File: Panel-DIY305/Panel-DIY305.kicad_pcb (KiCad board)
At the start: 2 copper layers, 62.2 x 39 mm, 400 parts

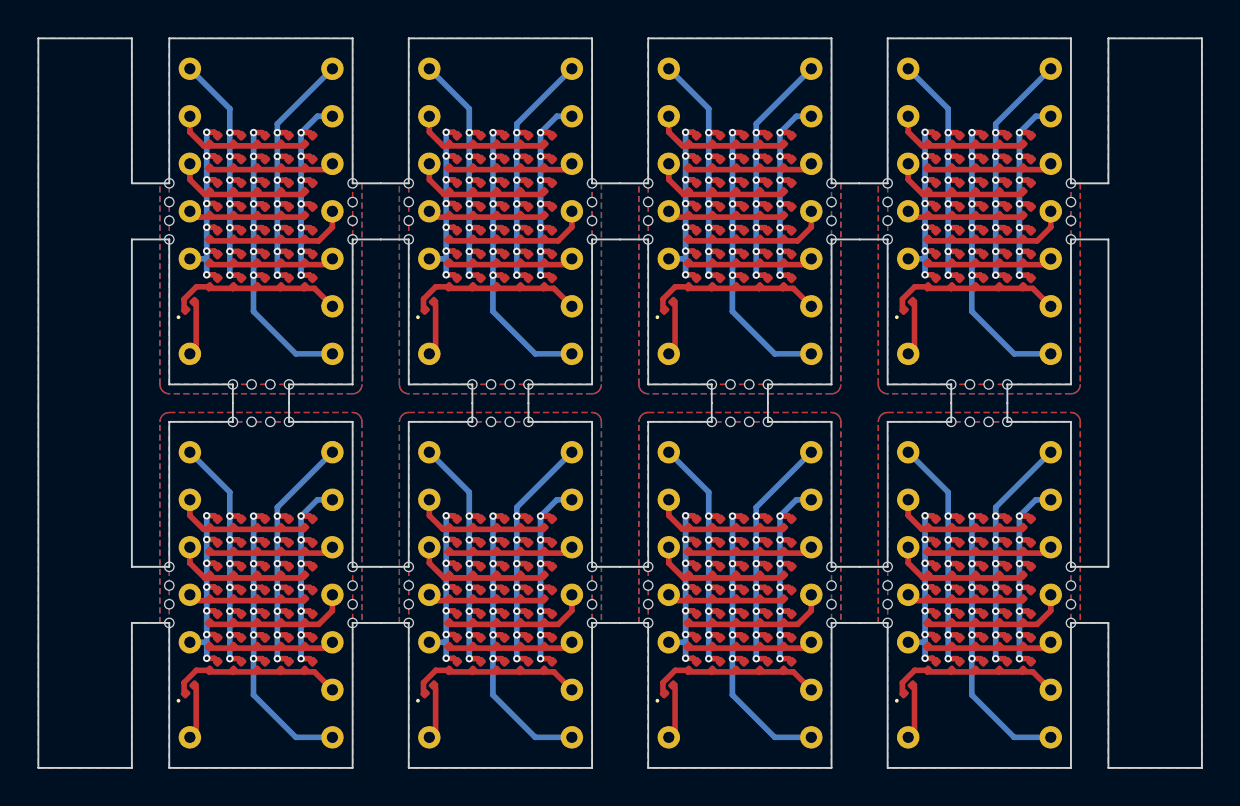
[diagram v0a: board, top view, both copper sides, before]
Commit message: Generated Panel
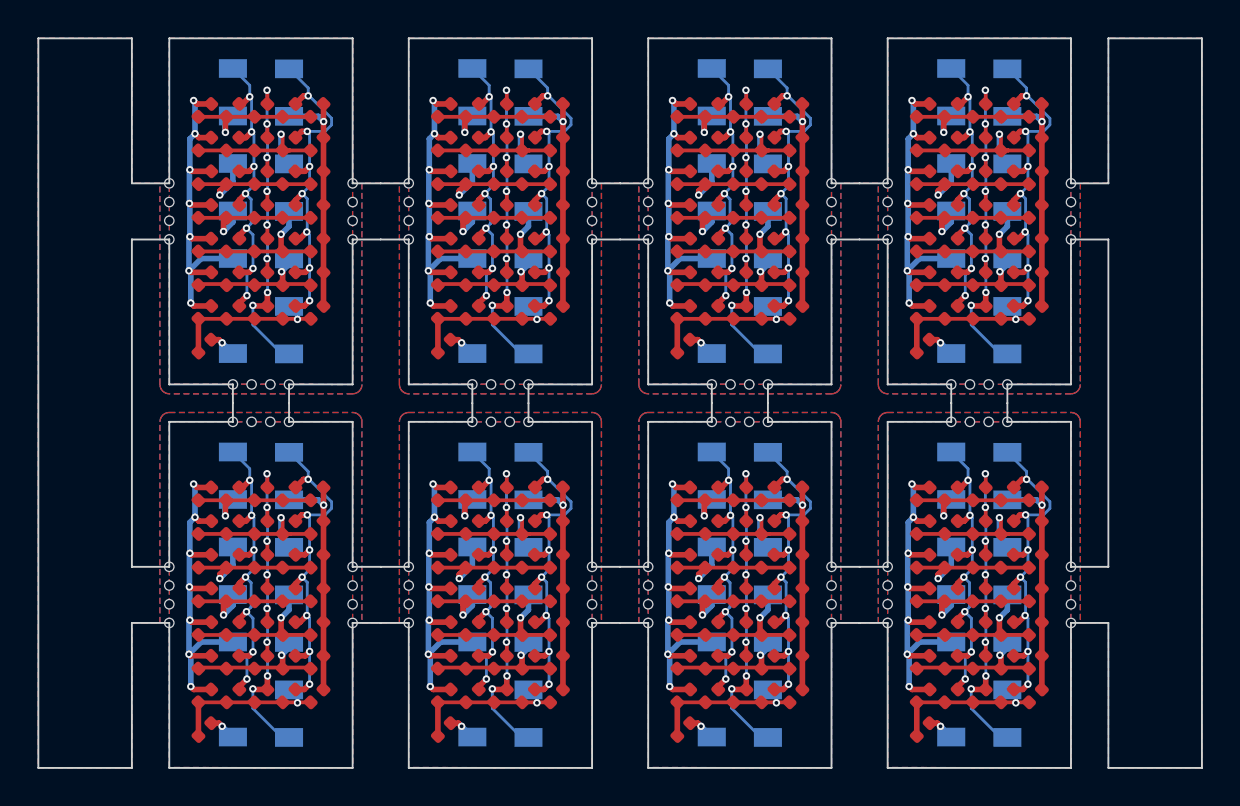
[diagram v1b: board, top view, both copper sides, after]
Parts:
- removed the D1 at (165.2, 25.4)
- removed the D1 at (165.2, 45.9)
- removed the D1 at (126.8, 45.9)
- removed the D1 at (152.4, 25.4)
- removed the D1 at (152.4, 45.9)
- removed the D1 at (139.6, 25.4)
- removed the D1 at (139.6, 45.9)
- removed the D1 at (126.8, 25.4)
- removed the D10 at (140.8, 48.5)
- removed the D10 at (128.0, 28.0)
- removed the D10 at (166.4, 28.0)
- removed the D10 at (153.6, 28.0)
- removed the D10 at (140.8, 28.0)
- removed the D10 at (166.4, 48.5)
- removed the D10 at (153.6, 48.5)
- removed the D10 at (128.0, 48.5)
- removed the D11 at (153.6, 49.7)
- removed the D11 at (166.4, 29.2)
- removed the D11 at (128.0, 29.2)
- removed the D11 at (140.8, 29.2)
- removed the D11 at (128.0, 49.7)
- removed the D11 at (140.8, 49.7)
- removed the D11 at (153.6, 29.2)
- removed the D11 at (166.4, 49.7)
- removed the D12 at (128.0, 30.5)
- removed the D12 at (140.8, 30.5)
- removed the D12 at (153.6, 30.5)
- removed the D12 at (166.4, 30.5)
- removed the D12 at (166.4, 51.0)
- removed the D12 at (140.8, 51.0)
- removed the D12 at (128.0, 51.0)
- removed the D12 at (153.6, 51.0)
- removed the D13 at (166.4, 31.8)
- removed the D13 at (166.4, 52.3)
- removed the D13 at (153.6, 31.8)
- removed the D13 at (140.8, 52.3)
- removed the D13 at (153.6, 52.3)
- removed the D13 at (128.0, 31.8)
- removed the D13 at (128.0, 52.3)
- removed the D13 at (140.8, 31.8)
- removed the D14 at (128.0, 53.6)
- removed the D14 at (153.6, 33.1)
- removed the D14 at (166.4, 53.6)
- removed the D14 at (128.0, 33.1)
- removed the D14 at (153.6, 53.6)
- removed the D14 at (140.8, 53.6)
- removed the D14 at (166.4, 33.1)
- removed the D14 at (140.8, 33.1)
- removed the D15 at (167.7, 25.4)
- removed the D15 at (129.3, 45.9)
- removed the D15 at (154.9, 45.9)
- removed the D15 at (154.9, 25.4)
- removed the D15 at (167.7, 45.9)
- removed the D15 at (142.1, 45.9)
- removed the D15 at (129.3, 25.4)
- removed the D15 at (142.1, 25.4)
- removed the D16 at (154.9, 26.7)
- removed the D16 at (142.1, 26.7)
- removed the D16 at (167.7, 26.7)
- removed the D16 at (129.3, 47.2)
- removed the D16 at (154.9, 47.2)
- removed the D16 at (129.3, 26.7)
- removed the D16 at (167.7, 47.2)
- removed the D16 at (142.1, 47.2)
- removed the D17 at (129.3, 28.0)
- removed the D17 at (167.7, 28.0)
- removed the D17 at (154.9, 28.0)
- removed the D17 at (142.1, 48.5)
- removed the D17 at (167.7, 48.5)
- removed the D17 at (142.1, 28.0)
- removed the D17 at (129.3, 48.5)
- removed the D17 at (154.9, 48.5)
- removed the D18 at (167.7, 49.7)
- removed the D18 at (167.7, 29.2)
- removed the D18 at (129.3, 49.7)
- removed the D18 at (142.1, 49.7)
- removed the D18 at (129.3, 29.2)
- removed the D18 at (142.1, 29.2)
- removed the D18 at (154.9, 29.2)
- removed the D18 at (154.9, 49.7)
- removed the D19 at (142.1, 51.0)
- removed the D19 at (129.3, 51.0)
- removed the D19 at (142.1, 30.5)
- removed the D19 at (167.7, 51.0)
- removed the D19 at (154.9, 51.0)
- removed the D19 at (154.9, 30.5)
- removed the D19 at (129.3, 30.5)
- removed the D19 at (167.7, 30.5)
- removed the D2 at (126.8, 26.7)
- removed the D2 at (126.8, 47.2)
- removed the D2 at (165.2, 26.7)
- removed the D2 at (165.2, 47.2)
- removed the D2 at (139.6, 47.2)
- removed the D2 at (139.6, 26.7)
- removed the D2 at (152.4, 26.7)
- removed the D2 at (152.4, 47.2)
- removed the D20 at (154.9, 31.8)
- removed the D20 at (154.9, 52.3)
- removed the D20 at (167.7, 52.3)
- removed the D20 at (129.3, 31.8)
- removed the D20 at (129.3, 52.3)
- removed the D20 at (142.1, 52.3)
- removed the D20 at (142.1, 31.8)
- removed the D20 at (167.7, 31.8)
- removed the D21 at (154.9, 33.1)
- removed the D21 at (167.7, 33.1)
- removed the D21 at (167.7, 53.6)
- removed the D21 at (129.3, 33.1)
- removed the D21 at (142.1, 53.6)
- removed the D21 at (129.3, 53.6)
- removed the D21 at (154.9, 53.6)
- removed the D21 at (142.1, 33.1)
- removed the D22 at (156.2, 25.4)
- removed the D22 at (143.4, 25.4)
- removed the D22 at (169.0, 25.4)
- removed the D22 at (156.2, 45.9)
- removed the D22 at (130.6, 45.9)
- removed the D22 at (130.6, 25.4)
- removed the D22 at (143.4, 45.9)
- removed the D22 at (169.0, 45.9)
- removed the D23 at (143.4, 26.7)
- removed the D23 at (156.2, 47.2)
- removed the D23 at (143.4, 47.2)
- removed the D23 at (156.2, 26.7)
- removed the D23 at (169.0, 26.7)
- removed the D23 at (169.0, 47.2)
- removed the D23 at (130.6, 47.2)
- removed the D23 at (130.6, 26.7)
- removed the D24 at (130.6, 28.0)
- removed the D24 at (169.0, 48.5)
- removed the D24 at (130.6, 48.5)
- removed the D24 at (143.4, 48.5)
- removed the D24 at (156.2, 28.0)
- removed the D24 at (156.2, 48.5)
- removed the D24 at (143.4, 28.0)
- removed the D24 at (169.0, 28.0)
- removed the D25 at (169.0, 49.7)
- removed the D25 at (156.2, 49.7)
- removed the D25 at (143.4, 49.7)
- removed the D25 at (143.4, 29.2)
- removed the D25 at (130.6, 29.2)
- removed the D25 at (156.2, 29.2)
- removed the D25 at (130.6, 49.7)
- removed the D25 at (169.0, 29.2)
- removed the D26 at (143.4, 30.5)
- removed the D26 at (156.2, 30.5)
- removed the D26 at (130.6, 51.0)
- removed the D26 at (143.4, 51.0)
- removed the D26 at (156.2, 51.0)
- removed the D26 at (169.0, 51.0)
- removed the D26 at (169.0, 30.5)
- removed the D26 at (130.6, 30.5)
- removed the D27 at (156.2, 52.3)
- removed the D27 at (130.6, 52.3)
- removed the D27 at (169.0, 31.8)
- removed the D27 at (130.6, 31.8)
- removed the D27 at (169.0, 52.3)
- removed the D27 at (143.4, 31.8)
- removed the D27 at (156.2, 31.8)
- removed the D27 at (143.4, 52.3)
- removed the D28 at (156.2, 53.6)
- removed the D28 at (130.6, 33.1)
- removed the D28 at (169.0, 53.6)
- removed the D28 at (156.2, 33.1)
- removed the D28 at (130.6, 53.6)
- removed the D28 at (169.0, 33.1)
- removed the D28 at (143.4, 33.1)
- removed the D28 at (143.4, 53.6)
- removed the D29 at (144.7, 45.9)
- removed the D29 at (144.7, 25.4)
- removed the D29 at (157.4, 45.9)
- removed the D29 at (131.8, 45.9)
- removed the D29 at (157.4, 25.4)
- removed the D29 at (131.8, 25.4)
- removed the D29 at (170.2, 25.4)
- removed the D29 at (170.2, 45.9)
- removed the D3 at (126.8, 28.0)
- removed the D3 at (165.2, 28.0)
- removed the D3 at (165.2, 48.5)
- removed the D3 at (152.4, 28.0)
- removed the D3 at (126.8, 48.5)
- removed the D3 at (139.6, 48.5)
- removed the D3 at (139.6, 28.0)
- removed the D3 at (152.4, 48.5)
- removed the D30 at (131.8, 47.2)
- removed the D30 at (170.2, 26.7)
- removed the D30 at (157.4, 26.7)
- removed the D30 at (131.8, 26.7)
- removed the D30 at (144.7, 47.2)
- removed the D30 at (157.4, 47.2)
- removed the D30 at (170.2, 47.2)
- removed the D30 at (144.7, 26.7)
- removed the D31 at (170.2, 48.5)
- removed the D31 at (144.7, 28.0)
- removed the D31 at (170.2, 28.0)
- removed the D31 at (157.4, 48.5)
- removed the D31 at (157.4, 28.0)
- removed the D31 at (144.7, 48.5)
- removed the D31 at (131.8, 48.5)
- removed the D31 at (131.8, 28.0)
- removed the D32 at (144.7, 29.2)
- removed the D32 at (157.4, 49.7)
- removed the D32 at (131.8, 29.2)
- removed the D32 at (157.4, 29.2)
- removed the D32 at (131.8, 49.7)
- removed the D32 at (144.7, 49.7)
- removed the D32 at (170.2, 29.2)
- removed the D32 at (170.2, 49.7)
- removed the D33 at (131.8, 51.0)
- removed the D33 at (144.7, 30.5)
- removed the D33 at (131.8, 30.5)
- removed the D33 at (157.4, 51.0)
- removed the D33 at (157.4, 30.5)
- removed the D33 at (170.2, 51.0)
- removed the D33 at (170.2, 30.5)
- removed the D33 at (144.7, 51.0)
- removed the D34 at (144.7, 52.3)
- removed the D34 at (144.7, 31.8)
- removed the D34 at (157.4, 52.3)
- removed the D34 at (170.2, 31.8)
- removed the D34 at (131.8, 52.3)
- removed the D34 at (131.8, 31.8)
- removed the D34 at (170.2, 52.3)
- removed the D34 at (157.4, 31.8)
- removed the D35 at (144.7, 53.6)
- removed the D35 at (157.4, 33.1)
- removed the D35 at (131.8, 33.1)
- removed the D35 at (144.7, 33.1)
- removed the D35 at (131.8, 53.6)
- removed the D35 at (157.4, 53.6)
- removed the D35 at (170.2, 33.1)
- removed the D35 at (170.2, 53.6)
- removed the D36 at (163.9, 34.3)
- removed the D36 at (151.1, 54.8)
- removed the D36 at (163.9, 54.8)
- removed the D36 at (125.5, 54.8)
- removed the D36 at (138.3, 54.8)
- removed the D36 at (151.1, 34.3)
- removed the D36 at (138.3, 34.3)
- removed the D36 at (125.5, 34.3)
- removed the D4 at (126.8, 29.2)
- removed the D4 at (165.2, 49.7)
- removed the D4 at (152.4, 29.2)
- removed the D4 at (139.6, 29.2)
- removed the D4 at (152.4, 49.7)
- removed the D4 at (165.2, 29.2)
- removed the D4 at (139.6, 49.7)
- removed the D4 at (126.8, 49.7)
- removed the D5 at (139.6, 30.5)
- removed the D5 at (139.6, 51.0)
- removed the D5 at (126.8, 51.0)
- removed the D5 at (152.4, 51.0)
- removed the D5 at (152.4, 30.5)
- removed the D5 at (126.8, 30.5)
- removed the D5 at (165.2, 51.0)
- removed the D5 at (165.2, 30.5)
- removed the D6 at (165.2, 52.3)
- removed the D6 at (152.4, 52.3)
- removed the D6 at (126.8, 31.8)
- removed the D6 at (152.4, 31.8)
- removed the D6 at (126.8, 52.3)
- removed the D6 at (165.2, 31.8)
- removed the D6 at (139.6, 52.3)
- removed the D6 at (139.6, 31.8)
- removed the D7 at (126.8, 33.1)
- removed the D7 at (139.6, 53.6)
- removed the D7 at (165.2, 33.1)
- removed the D7 at (126.8, 53.6)
- removed the D7 at (165.2, 53.6)
- removed the D7 at (139.6, 33.1)
- removed the D7 at (152.4, 33.1)
- removed the D7 at (152.4, 53.6)
- removed the D8 at (153.6, 45.9)
- removed the D8 at (153.6, 25.4)
- removed the D8 at (128.0, 25.4)
- removed the D8 at (140.8, 45.9)
- removed the D8 at (128.0, 45.9)
- removed the D8 at (166.4, 25.4)
- removed the D8 at (166.4, 45.9)
- removed the D8 at (140.8, 25.4)
- removed the D9 at (128.0, 26.7)
- removed the D9 at (166.4, 26.7)
- removed the D9 at (140.8, 26.7)
- removed the D9 at (128.0, 47.2)
- removed the D9 at (153.6, 47.2)
- removed the D9 at (140.8, 47.2)
- removed the D9 at (153.6, 26.7)
- removed the D9 at (166.4, 47.2)
- removed G*** (x8): LOGO, LOGO
- removed J4 (x8): , Package_DIP:DIP-14_W7.62mm
- added D1: LED, LED_SMD:LED_0402_1005Metric, F.Cu at (139.1, 44.4)
- added D1: LED, LED_SMD:LED_0402_1005Metric, F.Cu at (164.7, 44.4)
- added D1: LED, LED_SMD:LED_0402_1005Metric, F.Cu at (151.9, 23.9)
- added D1: LED, LED_SMD:LED_0402_1005Metric, F.Cu at (151.9, 44.4)
- added D1: LED, LED_SMD:LED_0402_1005Metric, F.Cu at (126.3, 23.9)
- added D1: LED, LED_SMD:LED_0402_1005Metric, F.Cu at (126.3, 44.4)
- added D1: LED, LED_SMD:LED_0402_1005Metric, F.Cu at (164.7, 23.9)
- added D1: LED, LED_SMD:LED_0402_1005Metric, F.Cu at (139.1, 23.9)
- added D10: LED, LED_SMD:LED_0402_1005Metric, F.Cu at (166.2, 27.4)
- added D10: LED, LED_SMD:LED_0402_1005Metric, F.Cu at (140.6, 27.4)
- added D10: LED, LED_SMD:LED_0402_1005Metric, F.Cu at (140.6, 48.0)
- added D10: LED, LED_SMD:LED_0402_1005Metric, F.Cu at (166.2, 48.0)
- added D10: LED, LED_SMD:LED_0402_1005Metric, F.Cu at (153.4, 48.0)
- added D10: LED, LED_SMD:LED_0402_1005Metric, F.Cu at (127.8, 27.4)
- added D10: LED, LED_SMD:LED_0402_1005Metric, F.Cu at (153.4, 27.4)
- added D10: LED, LED_SMD:LED_0402_1005Metric, F.Cu at (127.8, 48.0)
- added D11: LED, LED_SMD:LED_0402_1005Metric, F.Cu at (140.6, 29.2)
- added D11: LED, LED_SMD:LED_0402_1005Metric, F.Cu at (140.6, 49.8)
- added D11: LED, LED_SMD:LED_0402_1005Metric, F.Cu at (153.4, 29.2)
- added D11: LED, LED_SMD:LED_0402_1005Metric, F.Cu at (127.8, 49.8)
- added D11: LED, LED_SMD:LED_0402_1005Metric, F.Cu at (153.4, 49.8)
- added D11: LED, LED_SMD:LED_0402_1005Metric, F.Cu at (166.2, 49.8)
- added D11: LED, LED_SMD:LED_0402_1005Metric, F.Cu at (166.2, 29.2)
- added D11: LED, LED_SMD:LED_0402_1005Metric, F.Cu at (127.8, 29.2)
- added D12: LED, LED_SMD:LED_0402_1005Metric, F.Cu at (166.2, 51.5)
- added D12: LED, LED_SMD:LED_0402_1005Metric, F.Cu at (140.6, 51.5)
- added D12: LED, LED_SMD:LED_0402_1005Metric, F.Cu at (140.6, 31.1)
- added D12: LED, LED_SMD:LED_0402_1005Metric, F.Cu at (153.4, 51.5)
- added D12: LED, LED_SMD:LED_0402_1005Metric, F.Cu at (166.2, 31.1)
- added D12: LED, LED_SMD:LED_0402_1005Metric, F.Cu at (153.4, 31.1)
- added D12: LED, LED_SMD:LED_0402_1005Metric, F.Cu at (127.8, 51.5)
- added D12: LED, LED_SMD:LED_0402_1005Metric, F.Cu at (127.8, 31.1)
- added D13: LED, LED_SMD:LED_0402_1005Metric, F.Cu at (166.2, 53.4)
- added D13: LED, LED_SMD:LED_0402_1005Metric, F.Cu at (140.6, 53.4)
- added D13: LED, LED_SMD:LED_0402_1005Metric, F.Cu at (166.2, 32.9)
- added D13: LED, LED_SMD:LED_0402_1005Metric, F.Cu at (127.8, 32.9)
- added D13: LED, LED_SMD:LED_0402_1005Metric, F.Cu at (153.4, 53.4)
- added D13: LED, LED_SMD:LED_0402_1005Metric, F.Cu at (127.8, 53.4)
- added D13: LED, LED_SMD:LED_0402_1005Metric, F.Cu at (140.6, 32.9)
- added D13: LED, LED_SMD:LED_0402_1005Metric, F.Cu at (153.4, 32.9)
- added D14: LED, LED_SMD:LED_0402_1005Metric, F.Cu at (127.8, 55.1)
- added D14: LED, LED_SMD:LED_0402_1005Metric, F.Cu at (140.6, 34.6)
- added D14: LED, LED_SMD:LED_0402_1005Metric, F.Cu at (127.8, 34.6)
- added D14: LED, LED_SMD:LED_0402_1005Metric, F.Cu at (166.2, 55.1)
- added D14: LED, LED_SMD:LED_0402_1005Metric, F.Cu at (140.6, 55.1)
- added D14: LED, LED_SMD:LED_0402_1005Metric, F.Cu at (166.2, 34.6)
- added D14: LED, LED_SMD:LED_0402_1005Metric, F.Cu at (153.4, 55.1)
- added D14: LED, LED_SMD:LED_0402_1005Metric, F.Cu at (153.4, 34.6)
- added D15: LED, LED_SMD:LED_0402_1005Metric, F.Cu at (167.7, 44.4)
- added D15: LED, LED_SMD:LED_0402_1005Metric, F.Cu at (142.1, 23.9)
- added D15: LED, LED_SMD:LED_0402_1005Metric, F.Cu at (129.3, 44.4)
- added D15: LED, LED_SMD:LED_0402_1005Metric, F.Cu at (129.3, 23.9)
- added D15: LED, LED_SMD:LED_0402_1005Metric, F.Cu at (154.9, 23.9)
- added D15: LED, LED_SMD:LED_0402_1005Metric, F.Cu at (154.9, 44.4)
- added D15: LED, LED_SMD:LED_0402_1005Metric, F.Cu at (167.7, 23.9)
- added D15: LED, LED_SMD:LED_0402_1005Metric, F.Cu at (142.1, 44.4)
- added D16: LED, LED_SMD:LED_0402_1005Metric, F.Cu at (154.9, 25.6)
- added D16: LED, LED_SMD:LED_0402_1005Metric, F.Cu at (129.3, 46.1)
- added D16: LED, LED_SMD:LED_0402_1005Metric, F.Cu at (142.1, 46.1)
- added D16: LED, LED_SMD:LED_0402_1005Metric, F.Cu at (129.3, 25.6)
- added D16: LED, LED_SMD:LED_0402_1005Metric, F.Cu at (167.7, 46.1)
- added D16: LED, LED_SMD:LED_0402_1005Metric, F.Cu at (167.7, 25.6)
- added D16: LED, LED_SMD:LED_0402_1005Metric, F.Cu at (154.9, 46.1)
- added D16: LED, LED_SMD:LED_0402_1005Metric, F.Cu at (142.1, 25.6)
- added D17: LED, LED_SMD:LED_0402_1005Metric, F.Cu at (129.3, 48.0)
- added D17: LED, LED_SMD:LED_0402_1005Metric, F.Cu at (154.9, 27.4)
- added D17: LED, LED_SMD:LED_0402_1005Metric, F.Cu at (167.7, 48.0)
- added D17: LED, LED_SMD:LED_0402_1005Metric, F.Cu at (154.9, 48.0)
- added D17: LED, LED_SMD:LED_0402_1005Metric, F.Cu at (129.3, 27.4)
- added D17: LED, LED_SMD:LED_0402_1005Metric, F.Cu at (167.7, 27.4)
- added D17: LED, LED_SMD:LED_0402_1005Metric, F.Cu at (142.1, 48.0)
- added D17: LED, LED_SMD:LED_0402_1005Metric, F.Cu at (142.1, 27.4)
- added D18: LED, LED_SMD:LED_0402_1005Metric, F.Cu at (142.1, 29.2)
- added D18: LED, LED_SMD:LED_0402_1005Metric, F.Cu at (167.7, 49.8)
- added D18: LED, LED_SMD:LED_0402_1005Metric, F.Cu at (129.3, 29.2)
- added D18: LED, LED_SMD:LED_0402_1005Metric, F.Cu at (167.7, 29.2)
- added D18: LED, LED_SMD:LED_0402_1005Metric, F.Cu at (142.1, 49.8)
- added D18: LED, LED_SMD:LED_0402_1005Metric, F.Cu at (154.9, 49.8)
- added D18: LED, LED_SMD:LED_0402_1005Metric, F.Cu at (154.9, 29.2)
- added D18: LED, LED_SMD:LED_0402_1005Metric, F.Cu at (129.3, 49.8)
- added D19: LED, LED_SMD:LED_0402_1005Metric, F.Cu at (167.7, 51.5)
- added D19: LED, LED_SMD:LED_0402_1005Metric, F.Cu at (129.3, 31.1)
- added D19: LED, LED_SMD:LED_0402_1005Metric, F.Cu at (142.1, 51.5)
- added D19: LED, LED_SMD:LED_0402_1005Metric, F.Cu at (167.7, 31.1)
- added D19: LED, LED_SMD:LED_0402_1005Metric, F.Cu at (142.1, 31.1)
- added D19: LED, LED_SMD:LED_0402_1005Metric, F.Cu at (129.3, 51.5)
- added D19: LED, LED_SMD:LED_0402_1005Metric, F.Cu at (154.9, 51.5)
- added D19: LED, LED_SMD:LED_0402_1005Metric, F.Cu at (154.9, 31.1)
- added D2: LED, LED_SMD:LED_0402_1005Metric, F.Cu at (126.3, 25.6)
- added D2: LED, LED_SMD:LED_0402_1005Metric, F.Cu at (151.9, 46.1)
- added D2: LED, LED_SMD:LED_0402_1005Metric, F.Cu at (164.7, 46.1)
- added D2: LED, LED_SMD:LED_0402_1005Metric, F.Cu at (126.3, 46.1)
- added D2: LED, LED_SMD:LED_0402_1005Metric, F.Cu at (151.9, 25.6)
- added D2: LED, LED_SMD:LED_0402_1005Metric, F.Cu at (139.1, 25.6)
- added D2: LED, LED_SMD:LED_0402_1005Metric, F.Cu at (164.7, 25.6)
- added D2: LED, LED_SMD:LED_0402_1005Metric, F.Cu at (139.1, 46.1)
- added D20: LED, LED_SMD:LED_0402_1005Metric, F.Cu at (142.1, 32.9)
- added D20: LED, LED_SMD:LED_0402_1005Metric, F.Cu at (154.9, 32.9)
- added D20: LED, LED_SMD:LED_0402_1005Metric, F.Cu at (129.3, 53.4)
- added D20: LED, LED_SMD:LED_0402_1005Metric, F.Cu at (154.9, 53.4)
- added D20: LED, LED_SMD:LED_0402_1005Metric, F.Cu at (129.3, 32.9)
- added D20: LED, LED_SMD:LED_0402_1005Metric, F.Cu at (167.7, 53.4)
- added D20: LED, LED_SMD:LED_0402_1005Metric, F.Cu at (142.1, 53.4)
- added D20: LED, LED_SMD:LED_0402_1005Metric, F.Cu at (167.7, 32.9)
- added D21: LED, LED_SMD:LED_0402_1005Metric, F.Cu at (167.7, 55.1)
- added D21: LED, LED_SMD:LED_0402_1005Metric, F.Cu at (167.7, 34.6)
- added D21: LED, LED_SMD:LED_0402_1005Metric, F.Cu at (142.1, 34.6)
- added D21: LED, LED_SMD:LED_0402_1005Metric, F.Cu at (129.3, 34.6)
- added D21: LED, LED_SMD:LED_0402_1005Metric, F.Cu at (129.3, 55.1)
- added D21: LED, LED_SMD:LED_0402_1005Metric, F.Cu at (154.9, 34.6)
- added D21: LED, LED_SMD:LED_0402_1005Metric, F.Cu at (154.9, 55.1)
- added D21: LED, LED_SMD:LED_0402_1005Metric, F.Cu at (142.1, 55.1)
- added D22: LED, LED_SMD:LED_0402_1005Metric, F.Cu at (130.8, 23.9)
- added D22: LED, LED_SMD:LED_0402_1005Metric, F.Cu at (143.6, 44.4)
- added D22: LED, LED_SMD:LED_0402_1005Metric, F.Cu at (169.2, 44.4)
- added D22: LED, LED_SMD:LED_0402_1005Metric, F.Cu at (130.8, 44.4)
- added D22: LED, LED_SMD:LED_0402_1005Metric, F.Cu at (156.4, 23.9)
- added D22: LED, LED_SMD:LED_0402_1005Metric, F.Cu at (169.2, 23.9)
- added D22: LED, LED_SMD:LED_0402_1005Metric, F.Cu at (143.6, 23.9)
- added D22: LED, LED_SMD:LED_0402_1005Metric, F.Cu at (156.4, 44.4)
- added D23: LED, LED_SMD:LED_0402_1005Metric, F.Cu at (143.6, 25.6)
- added D23: LED, LED_SMD:LED_0402_1005Metric, F.Cu at (156.4, 46.1)
- added D23: LED, LED_SMD:LED_0402_1005Metric, F.Cu at (130.8, 46.1)
- added D23: LED, LED_SMD:LED_0402_1005Metric, F.Cu at (130.8, 25.6)
- added D23: LED, LED_SMD:LED_0402_1005Metric, F.Cu at (143.6, 46.1)
- added D23: LED, LED_SMD:LED_0402_1005Metric, F.Cu at (169.2, 46.1)
- added D23: LED, LED_SMD:LED_0402_1005Metric, F.Cu at (169.2, 25.6)
- added D23: LED, LED_SMD:LED_0402_1005Metric, F.Cu at (156.4, 25.6)
- added D24: LED, LED_SMD:LED_0402_1005Metric, F.Cu at (156.4, 48.0)
- added D24: LED, LED_SMD:LED_0402_1005Metric, F.Cu at (143.6, 27.4)
- added D24: LED, LED_SMD:LED_0402_1005Metric, F.Cu at (143.6, 48.0)
- added D24: LED, LED_SMD:LED_0402_1005Metric, F.Cu at (130.8, 27.4)
- added D24: LED, LED_SMD:LED_0402_1005Metric, F.Cu at (169.2, 48.0)
- added D24: LED, LED_SMD:LED_0402_1005Metric, F.Cu at (169.2, 27.4)
- added D24: LED, LED_SMD:LED_0402_1005Metric, F.Cu at (156.4, 27.4)
- added D24: LED, LED_SMD:LED_0402_1005Metric, F.Cu at (130.8, 48.0)
- added D25: LED, LED_SMD:LED_0402_1005Metric, F.Cu at (130.8, 29.2)
- added D25: LED, LED_SMD:LED_0402_1005Metric, F.Cu at (156.4, 49.8)
- added D25: LED, LED_SMD:LED_0402_1005Metric, F.Cu at (143.6, 29.2)
- added D25: LED, LED_SMD:LED_0402_1005Metric, F.Cu at (143.6, 49.8)
- added D25: LED, LED_SMD:LED_0402_1005Metric, F.Cu at (169.2, 29.2)
- added D25: LED, LED_SMD:LED_0402_1005Metric, F.Cu at (156.4, 29.2)
- added D25: LED, LED_SMD:LED_0402_1005Metric, F.Cu at (130.8, 49.8)
- added D25: LED, LED_SMD:LED_0402_1005Metric, F.Cu at (169.2, 49.8)
- added D26: LED, LED_SMD:LED_0402_1005Metric, F.Cu at (156.4, 51.5)
- added D26: LED, LED_SMD:LED_0402_1005Metric, F.Cu at (143.6, 51.5)
- added D26: LED, LED_SMD:LED_0402_1005Metric, F.Cu at (156.4, 31.1)
- added D26: LED, LED_SMD:LED_0402_1005Metric, F.Cu at (130.8, 31.1)
- added D26: LED, LED_SMD:LED_0402_1005Metric, F.Cu at (169.2, 31.1)
- added D26: LED, LED_SMD:LED_0402_1005Metric, F.Cu at (130.8, 51.5)
- added D26: LED, LED_SMD:LED_0402_1005Metric, F.Cu at (169.2, 51.5)
- added D26: LED, LED_SMD:LED_0402_1005Metric, F.Cu at (143.6, 31.1)
- added D27: LED, LED_SMD:LED_0402_1005Metric, F.Cu at (156.4, 32.9)
- added D27: LED, LED_SMD:LED_0402_1005Metric, F.Cu at (169.2, 53.4)
- added D27: LED, LED_SMD:LED_0402_1005Metric, F.Cu at (143.6, 53.4)
- added D27: LED, LED_SMD:LED_0402_1005Metric, F.Cu at (130.8, 53.4)
- added D27: LED, LED_SMD:LED_0402_1005Metric, F.Cu at (156.4, 53.4)
- added D27: LED, LED_SMD:LED_0402_1005Metric, F.Cu at (169.2, 32.9)
- added D27: LED, LED_SMD:LED_0402_1005Metric, F.Cu at (143.6, 32.9)
- added D27: LED, LED_SMD:LED_0402_1005Metric, F.Cu at (130.8, 32.9)
- added D28: LED, LED_SMD:LED_0402_1005Metric, F.Cu at (130.8, 34.6)
- added D28: LED, LED_SMD:LED_0402_1005Metric, F.Cu at (156.4, 55.1)
- added D28: LED, LED_SMD:LED_0402_1005Metric, F.Cu at (143.6, 55.1)
- added D28: LED, LED_SMD:LED_0402_1005Metric, F.Cu at (169.2, 34.6)
- added D28: LED, LED_SMD:LED_0402_1005Metric, F.Cu at (169.2, 55.1)
- added D28: LED, LED_SMD:LED_0402_1005Metric, F.Cu at (130.8, 55.1)
- added D28: LED, LED_SMD:LED_0402_1005Metric, F.Cu at (143.6, 34.6)
- added D28: LED, LED_SMD:LED_0402_1005Metric, F.Cu at (156.4, 34.6)
- added D29: LED, LED_SMD:LED_0402_1005Metric, F.Cu at (157.9, 23.9)
- added D29: LED, LED_SMD:LED_0402_1005Metric, F.Cu at (145.1, 44.4)
- added D29: LED, LED_SMD:LED_0402_1005Metric, F.Cu at (145.1, 23.9)
- added D29: LED, LED_SMD:LED_0402_1005Metric, F.Cu at (157.9, 44.4)
- added D29: LED, LED_SMD:LED_0402_1005Metric, F.Cu at (132.3, 44.4)
- added D29: LED, LED_SMD:LED_0402_1005Metric, F.Cu at (132.3, 23.9)
- added D29: LED, LED_SMD:LED_0402_1005Metric, F.Cu at (170.7, 23.9)
- added D29: LED, LED_SMD:LED_0402_1005Metric, F.Cu at (170.7, 44.4)
- added D3: LED, LED_SMD:LED_0402_1005Metric, F.Cu at (164.7, 48.0)
- added D3: LED, LED_SMD:LED_0402_1005Metric, F.Cu at (126.3, 27.4)
- added D3: LED, LED_SMD:LED_0402_1005Metric, F.Cu at (126.3, 48.0)
- added D3: LED, LED_SMD:LED_0402_1005Metric, F.Cu at (139.1, 27.4)
- added D3: LED, LED_SMD:LED_0402_1005Metric, F.Cu at (164.7, 27.4)
- added D3: LED, LED_SMD:LED_0402_1005Metric, F.Cu at (151.9, 48.0)
- added D3: LED, LED_SMD:LED_0402_1005Metric, F.Cu at (139.1, 48.0)
- added D3: LED, LED_SMD:LED_0402_1005Metric, F.Cu at (151.9, 27.4)
- added D30: LED, LED_SMD:LED_0402_1005Metric, F.Cu at (132.3, 46.1)
- added D30: LED, LED_SMD:LED_0402_1005Metric, F.Cu at (157.9, 46.1)
- added D30: LED, LED_SMD:LED_0402_1005Metric, F.Cu at (145.1, 25.6)
- added D30: LED, LED_SMD:LED_0402_1005Metric, F.Cu at (132.3, 25.6)
- added D30: LED, LED_SMD:LED_0402_1005Metric, F.Cu at (145.1, 46.1)
- added D30: LED, LED_SMD:LED_0402_1005Metric, F.Cu at (170.7, 25.6)
- added D30: LED, LED_SMD:LED_0402_1005Metric, F.Cu at (157.9, 25.6)
- added D30: LED, LED_SMD:LED_0402_1005Metric, F.Cu at (170.7, 46.1)
- added D31: LED, LED_SMD:LED_0402_1005Metric, F.Cu at (132.3, 48.0)
- added D31: LED, LED_SMD:LED_0402_1005Metric, F.Cu at (157.9, 27.4)
- added D31: LED, LED_SMD:LED_0402_1005Metric, F.Cu at (145.1, 48.0)
- added D31: LED, LED_SMD:LED_0402_1005Metric, F.Cu at (170.7, 48.0)
- added D31: LED, LED_SMD:LED_0402_1005Metric, F.Cu at (157.9, 48.0)
- added D31: LED, LED_SMD:LED_0402_1005Metric, F.Cu at (170.7, 27.4)
- added D31: LED, LED_SMD:LED_0402_1005Metric, F.Cu at (132.3, 27.4)
- added D31: LED, LED_SMD:LED_0402_1005Metric, F.Cu at (145.1, 27.4)
- added D32: LED, LED_SMD:LED_0402_1005Metric, F.Cu at (145.1, 49.8)
- added D32: LED, LED_SMD:LED_0402_1005Metric, F.Cu at (145.1, 29.2)
- added D32: LED, LED_SMD:LED_0402_1005Metric, F.Cu at (170.7, 49.8)
- added D32: LED, LED_SMD:LED_0402_1005Metric, F.Cu at (132.3, 29.2)
- added D32: LED, LED_SMD:LED_0402_1005Metric, F.Cu at (157.9, 49.8)
- added D32: LED, LED_SMD:LED_0402_1005Metric, F.Cu at (157.9, 29.2)
- added D32: LED, LED_SMD:LED_0402_1005Metric, F.Cu at (132.3, 49.8)
- added D32: LED, LED_SMD:LED_0402_1005Metric, F.Cu at (170.7, 29.2)
- added D33: LED, LED_SMD:LED_0402_1005Metric, F.Cu at (145.1, 51.5)
- added D33: LED, LED_SMD:LED_0402_1005Metric, F.Cu at (157.9, 31.1)
- added D33: LED, LED_SMD:LED_0402_1005Metric, F.Cu at (170.7, 51.5)
- added D33: LED, LED_SMD:LED_0402_1005Metric, F.Cu at (132.3, 31.1)
- added D33: LED, LED_SMD:LED_0402_1005Metric, F.Cu at (170.7, 31.1)
- added D33: LED, LED_SMD:LED_0402_1005Metric, F.Cu at (132.3, 51.5)
- added D33: LED, LED_SMD:LED_0402_1005Metric, F.Cu at (145.1, 31.1)
- added D33: LED, LED_SMD:LED_0402_1005Metric, F.Cu at (157.9, 51.5)
- added D34: LED, LED_SMD:LED_0402_1005Metric, F.Cu at (145.1, 32.9)
- added D34: LED, LED_SMD:LED_0402_1005Metric, F.Cu at (157.9, 32.9)
- added D34: LED, LED_SMD:LED_0402_1005Metric, F.Cu at (170.7, 32.9)
- added D34: LED, LED_SMD:LED_0402_1005Metric, F.Cu at (157.9, 53.4)
- added D34: LED, LED_SMD:LED_0402_1005Metric, F.Cu at (132.3, 32.9)
- added D34: LED, LED_SMD:LED_0402_1005Metric, F.Cu at (145.1, 53.4)
- added D34: LED, LED_SMD:LED_0402_1005Metric, F.Cu at (170.7, 53.4)
- added D34: LED, LED_SMD:LED_0402_1005Metric, F.Cu at (132.3, 53.4)
- added D35: LED, LED_SMD:LED_0402_1005Metric, F.Cu at (132.3, 34.6)
- added D35: LED, LED_SMD:LED_0402_1005Metric, F.Cu at (132.3, 55.1)
- added D35: LED, LED_SMD:LED_0402_1005Metric, F.Cu at (170.7, 34.6)
- added D35: LED, LED_SMD:LED_0402_1005Metric, F.Cu at (157.9, 34.6)
- added D35: LED, LED_SMD:LED_0402_1005Metric, F.Cu at (157.9, 55.1)
- added D35: LED, LED_SMD:LED_0402_1005Metric, F.Cu at (145.1, 34.6)
- added D35: LED, LED_SMD:LED_0402_1005Metric, F.Cu at (145.1, 55.1)
- added D35: LED, LED_SMD:LED_0402_1005Metric, F.Cu at (170.7, 55.1)
- added D36: LED, LED_SMD:LED_0402_1005Metric, F.Cu at (139.1, 57.0)
- added D36: LED, LED_SMD:LED_0402_1005Metric, F.Cu at (126.3, 36.5)
- added D36: LED, LED_SMD:LED_0402_1005Metric, F.Cu at (139.1, 36.5)
- added D36: LED, LED_SMD:LED_0402_1005Metric, F.Cu at (126.3, 57.0)
- added D36: LED, LED_SMD:LED_0402_1005Metric, F.Cu at (164.7, 36.5)
- added D36: LED, LED_SMD:LED_0402_1005Metric, F.Cu at (164.7, 57.0)
- added D36: LED, LED_SMD:LED_0402_1005Metric, F.Cu at (151.9, 36.5)
- added D36: LED, LED_SMD:LED_0402_1005Metric, F.Cu at (151.9, 57.0)
- added D4: LED, LED_SMD:LED_0402_1005Metric, F.Cu at (139.1, 29.2)
- added D4: LED, LED_SMD:LED_0402_1005Metric, F.Cu at (126.3, 29.2)
- added D4: LED, LED_SMD:LED_0402_1005Metric, F.Cu at (126.3, 49.8)
- added D4: LED, LED_SMD:LED_0402_1005Metric, F.Cu at (164.7, 29.2)
- added D4: LED, LED_SMD:LED_0402_1005Metric, F.Cu at (164.7, 49.8)
- added D4: LED, LED_SMD:LED_0402_1005Metric, F.Cu at (151.9, 49.8)
- added D4: LED, LED_SMD:LED_0402_1005Metric, F.Cu at (151.9, 29.2)
- added D4: LED, LED_SMD:LED_0402_1005Metric, F.Cu at (139.1, 49.8)
- added D5: LED, LED_SMD:LED_0402_1005Metric, F.Cu at (139.1, 31.1)
- added D5: LED, LED_SMD:LED_0402_1005Metric, F.Cu at (139.1, 51.5)
- added D5: LED, LED_SMD:LED_0402_1005Metric, F.Cu at (164.7, 31.1)
- added D5: LED, LED_SMD:LED_0402_1005Metric, F.Cu at (164.7, 51.5)
- added D5: LED, LED_SMD:LED_0402_1005Metric, F.Cu at (126.3, 51.5)
- added D5: LED, LED_SMD:LED_0402_1005Metric, F.Cu at (126.3, 31.1)
- added D5: LED, LED_SMD:LED_0402_1005Metric, F.Cu at (151.9, 31.1)
- added D5: LED, LED_SMD:LED_0402_1005Metric, F.Cu at (151.9, 51.5)
- added D6: LED, LED_SMD:LED_0402_1005Metric, F.Cu at (126.3, 53.4)
- added D6: LED, LED_SMD:LED_0402_1005Metric, F.Cu at (164.7, 32.9)
- added D6: LED, LED_SMD:LED_0402_1005Metric, F.Cu at (139.1, 32.9)
- added D6: LED, LED_SMD:LED_0402_1005Metric, F.Cu at (126.3, 32.9)
- added D6: LED, LED_SMD:LED_0402_1005Metric, F.Cu at (151.9, 32.9)
- added D6: LED, LED_SMD:LED_0402_1005Metric, F.Cu at (164.7, 53.4)
- added D6: LED, LED_SMD:LED_0402_1005Metric, F.Cu at (139.1, 53.4)
- added D6: LED, LED_SMD:LED_0402_1005Metric, F.Cu at (151.9, 53.4)
- added D7: LED, LED_SMD:LED_0402_1005Metric, F.Cu at (126.3, 34.6)
- added D7: LED, LED_SMD:LED_0402_1005Metric, F.Cu at (126.3, 55.1)
- added D7: LED, LED_SMD:LED_0402_1005Metric, F.Cu at (139.1, 55.1)
- added D7: LED, LED_SMD:LED_0402_1005Metric, F.Cu at (151.9, 55.1)
- added D7: LED, LED_SMD:LED_0402_1005Metric, F.Cu at (164.7, 34.6)
- added D7: LED, LED_SMD:LED_0402_1005Metric, F.Cu at (139.1, 34.6)
- added D7: LED, LED_SMD:LED_0402_1005Metric, F.Cu at (164.7, 55.1)
- added D7: LED, LED_SMD:LED_0402_1005Metric, F.Cu at (151.9, 34.6)
- added D8: LED, LED_SMD:LED_0402_1005Metric, F.Cu at (166.2, 23.9)
- added D8: LED, LED_SMD:LED_0402_1005Metric, F.Cu at (127.8, 44.4)
- added D8: LED, LED_SMD:LED_0402_1005Metric, F.Cu at (153.4, 23.9)
- added D8: LED, LED_SMD:LED_0402_1005Metric, F.Cu at (127.8, 23.9)
- added D8: LED, LED_SMD:LED_0402_1005Metric, F.Cu at (153.4, 44.4)
- added D8: LED, LED_SMD:LED_0402_1005Metric, F.Cu at (140.6, 23.9)
- added D8: LED, LED_SMD:LED_0402_1005Metric, F.Cu at (166.2, 44.4)
- added D8: LED, LED_SMD:LED_0402_1005Metric, F.Cu at (140.6, 44.4)
- added D9: LED, LED_SMD:LED_0402_1005Metric, F.Cu at (166.2, 46.1)
- added D9: LED, LED_SMD:LED_0402_1005Metric, F.Cu at (127.8, 25.6)
- added D9: LED, LED_SMD:LED_0402_1005Metric, F.Cu at (153.4, 25.6)
- added D9: LED, LED_SMD:LED_0402_1005Metric, F.Cu at (153.4, 46.1)
- added D9: LED, LED_SMD:LED_0402_1005Metric, F.Cu at (127.8, 46.1)
- added D9: LED, LED_SMD:LED_0402_1005Metric, F.Cu at (166.2, 25.6)
- added D9: LED, LED_SMD:LED_0402_1005Metric, F.Cu at (140.6, 46.1)
- added D9: LED, LED_SMD:LED_0402_1005Metric, F.Cu at (140.6, 25.6)
- added REF**: PinHeader_2x07_P2.54mm_Vertical_SMD, Connector_PinHeader_2.54mm:PinHeader_2x07_P2.54mm_Vertical_SMD, B.Cu at (142.1, 49.8)
- added REF**: PinHeader_2x07_P2.54mm_Vertical_SMD, Connector_PinHeader_2.54mm:PinHeader_2x07_P2.54mm_Vertical_SMD, B.Cu at (154.9, 29.2)
- added REF**: PinHeader_2x07_P2.54mm_Vertical_SMD, Connector_PinHeader_2.54mm:PinHeader_2x07_P2.54mm_Vertical_SMD, B.Cu at (154.9, 49.8)
- added REF**: PinHeader_2x07_P2.54mm_Vertical_SMD, Connector_PinHeader_2.54mm:PinHeader_2x07_P2.54mm_Vertical_SMD, B.Cu at (129.3, 29.2)
- added REF**: PinHeader_2x07_P2.54mm_Vertical_SMD, Connector_PinHeader_2.54mm:PinHeader_2x07_P2.54mm_Vertical_SMD, B.Cu at (129.3, 49.8)
- added REF**: PinHeader_2x07_P2.54mm_Vertical_SMD, Connector_PinHeader_2.54mm:PinHeader_2x07_P2.54mm_Vertical_SMD, B.Cu at (167.7, 29.2)
- added REF**: PinHeader_2x07_P2.54mm_Vertical_SMD, Connector_PinHeader_2.54mm:PinHeader_2x07_P2.54mm_Vertical_SMD, B.Cu at (167.7, 49.8)
- added REF**: PinHeader_2x07_P2.54mm_Vertical_SMD, Connector_PinHeader_2.54mm:PinHeader_2x07_P2.54mm_Vertical_SMD, B.Cu at (142.1, 29.2)
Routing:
- net Board_4-C1: track 13.2 -> 21.6 mm
- net Board_0-C1: track 13.2 -> 21.6 mm
- net Board_7-C1: track 13.2 -> 21.6 mm
- net Board_3-C1: track 13.2 -> 21.6 mm
- net Board_6-C1: track 13.2 -> 21.6 mm
- net Board_2-C1: track 13.2 -> 21.6 mm
- net Board_5-C1: track 13.2 -> 21.6 mm
- net Board_1-C1: track 13.2 -> 21.6 mm
- net Board_6-R3: track 16.9 -> 8.70 mm, vias 0 -> 1
- net Board_2-R3: track 16.9 -> 8.70 mm, vias 0 -> 1
- net Board_5-R3: track 16.9 -> 8.70 mm, vias 0 -> 1
- net Board_4-R3: track 16.9 -> 8.70 mm, vias 0 -> 1
- net Board_1-R3: track 16.9 -> 8.70 mm, vias 0 -> 1
- net Board_0-R3: track 16.9 -> 8.70 mm, vias 0 -> 1
- net Board_7-R3: track 16.9 -> 8.70 mm, vias 0 -> 1
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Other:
- board text removed: "D8"
- board text removed: "JLCJLCJLCJLC"
